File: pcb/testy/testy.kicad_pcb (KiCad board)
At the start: 2 copper layers, 175 x 108 mm, 84 parts, among them SW3:1 PG1511_socket, U1 ProMicro

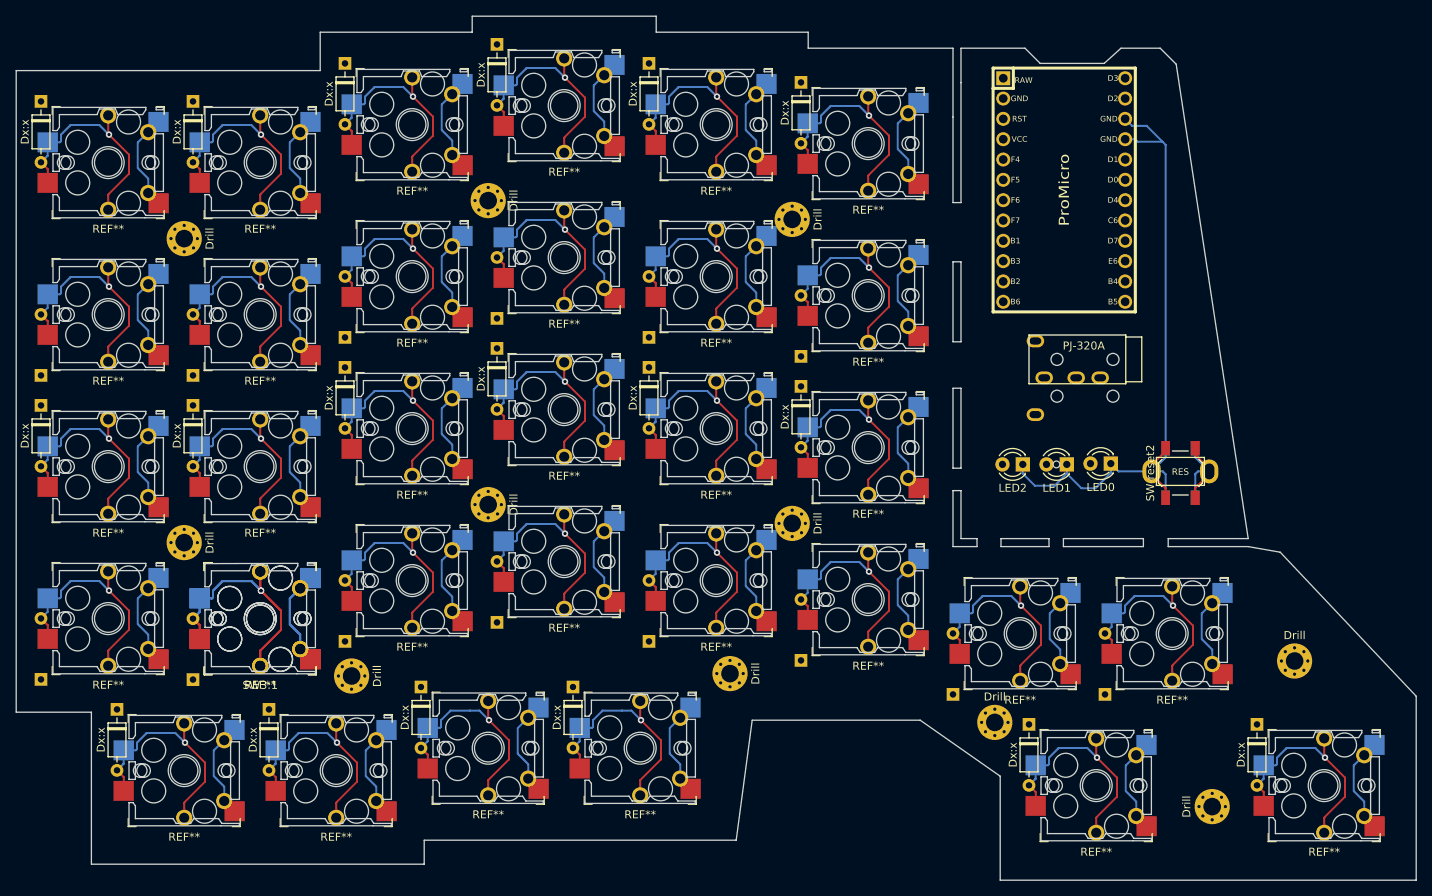
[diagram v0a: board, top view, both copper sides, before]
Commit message: feat: some more layout
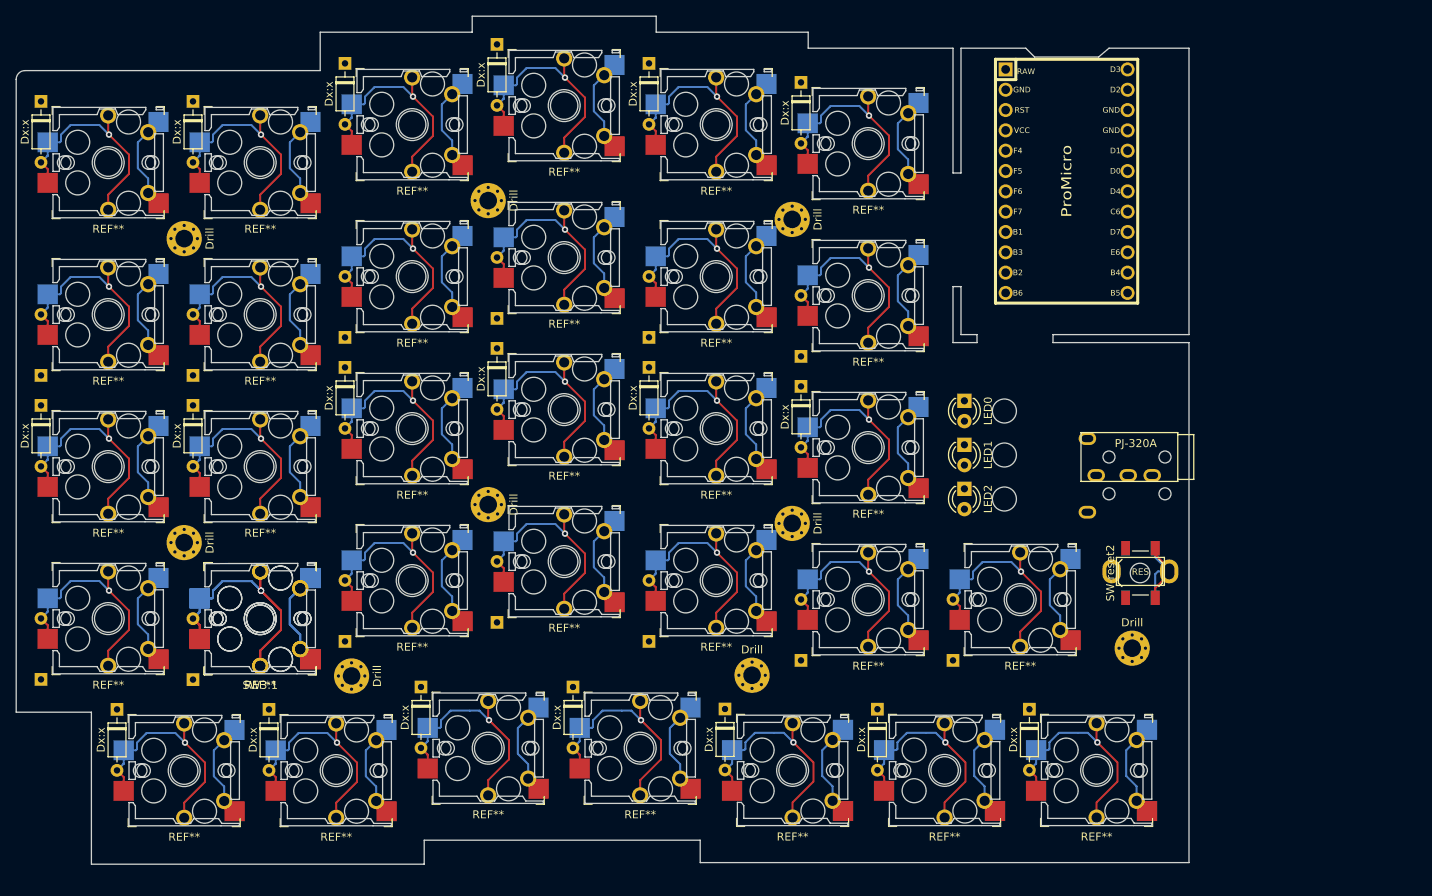
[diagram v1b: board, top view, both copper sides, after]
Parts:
- removed the Drill at (220.2, 141.8)
- removed the Drill at (230.5, 123.6)
- Dx:x: moved to F.Cu
- moved REF** 50.4 mm to (167.8, 137.3)
- moved Drill 50.4 mm to (210.2, 122.0), turned to 0 degrees
- moved Dx:x 47.5 mm to (159.3, 129.6), turned to 270 degrees
- moved Dx:x 47.5 mm to (178.3, 129.6)
- moved REF** 47.5 mm to (186.8, 137.3)
- moved Drill 30.9 mm to (162.7, 125.4)
- moved LED0 19.9 mm to (189.2, 91.1), turned to 270 degrees
- moved TRRS1 13.8 mm to (215.9, 100.4)
- moved SW-reset1 13.5 mm to (211.2, 114.2)
- moved SW-reset2 13.5 mm to (211.2, 112.6)
- moved SW-reset3 13.5 mm to (211.2, 112.6)
- moved LED1 13.0 mm to (189.2, 96.6), turned to 270 degrees
- moved LED2 7.91 mm to (189.2, 102.1), turned to 270 degrees
- moved Dx:x 4.25 mm to (187.8, 123.5)
- moved REF** 4.25 mm to (196.2, 115.9)
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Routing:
- net GND: track 88.0 -> 0.00 mm
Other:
- board size 175 x 108 mm -> 146.6 x 106 mm
- board text added: "TODO add OLED headers"
- board text removed: "<--- Should we have centered holes to make drilling easier?"
